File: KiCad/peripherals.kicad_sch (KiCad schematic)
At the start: 36 parts, among them IC1 MIC5350-SGYMT-TR, J1 Conn_02x06_Counter_Clockwise, J2 USB_C_Receptacle_USB2.0_14P, J3 Conn_01x07, J4 Conn_01x06, J6 Conn_02x11_Counter_Clockwise, U1 EM008LX, U2 EM008LX, U3 EM008LX, X1 2x5 0.05" SWD

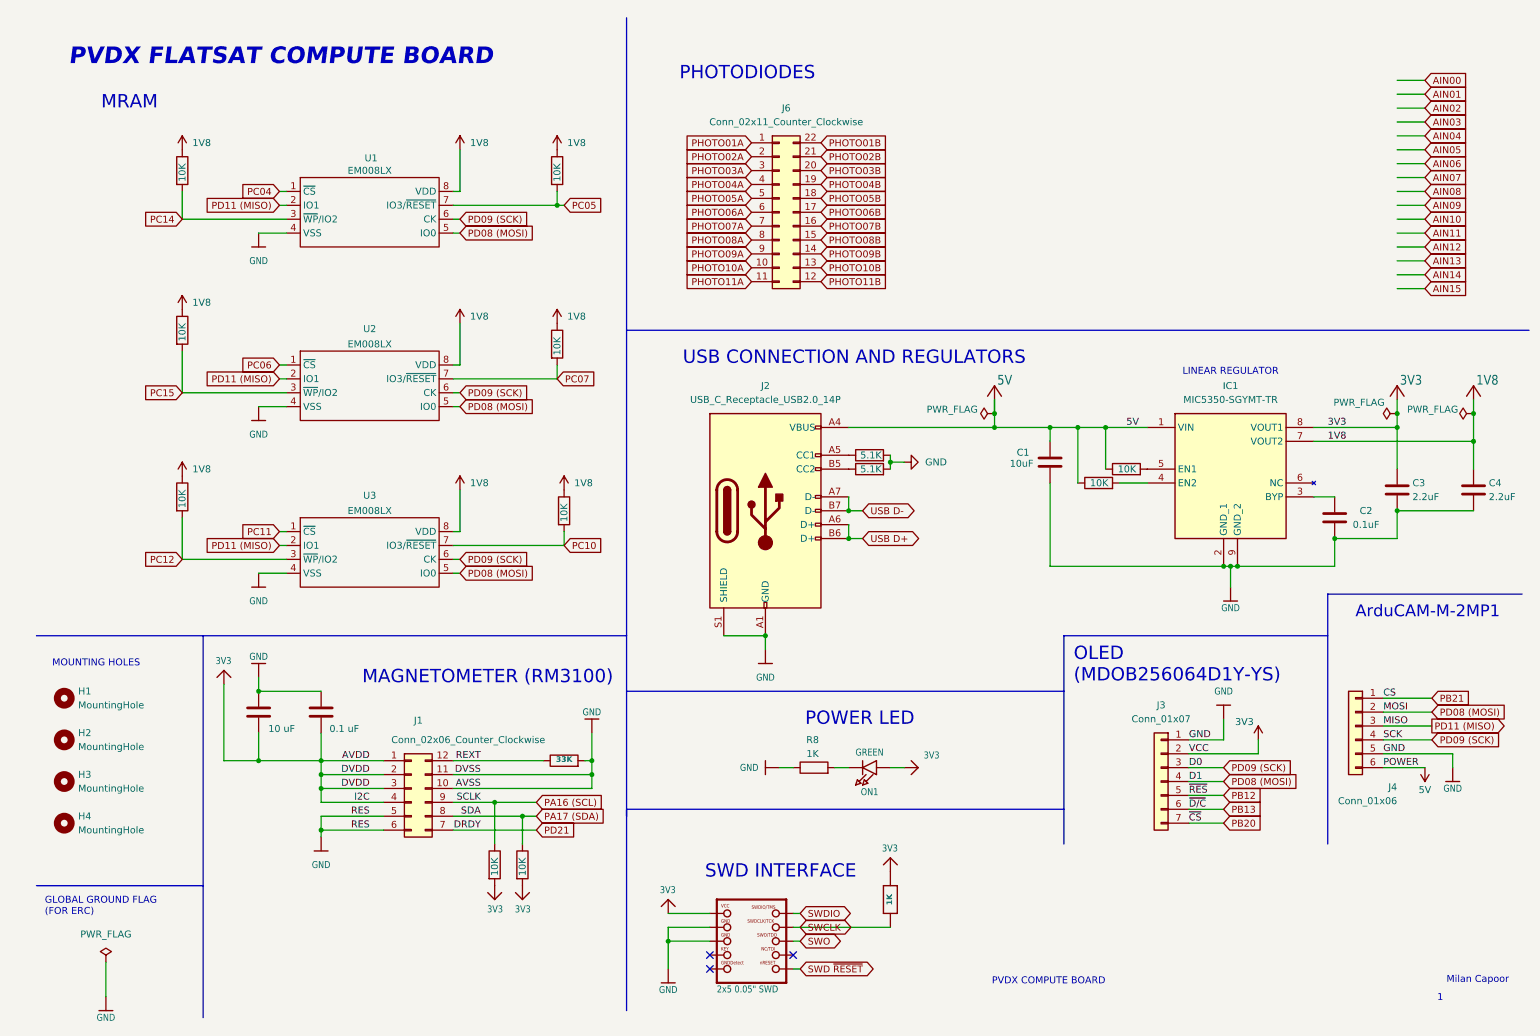
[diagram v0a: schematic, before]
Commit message: update draft to 11/13 version
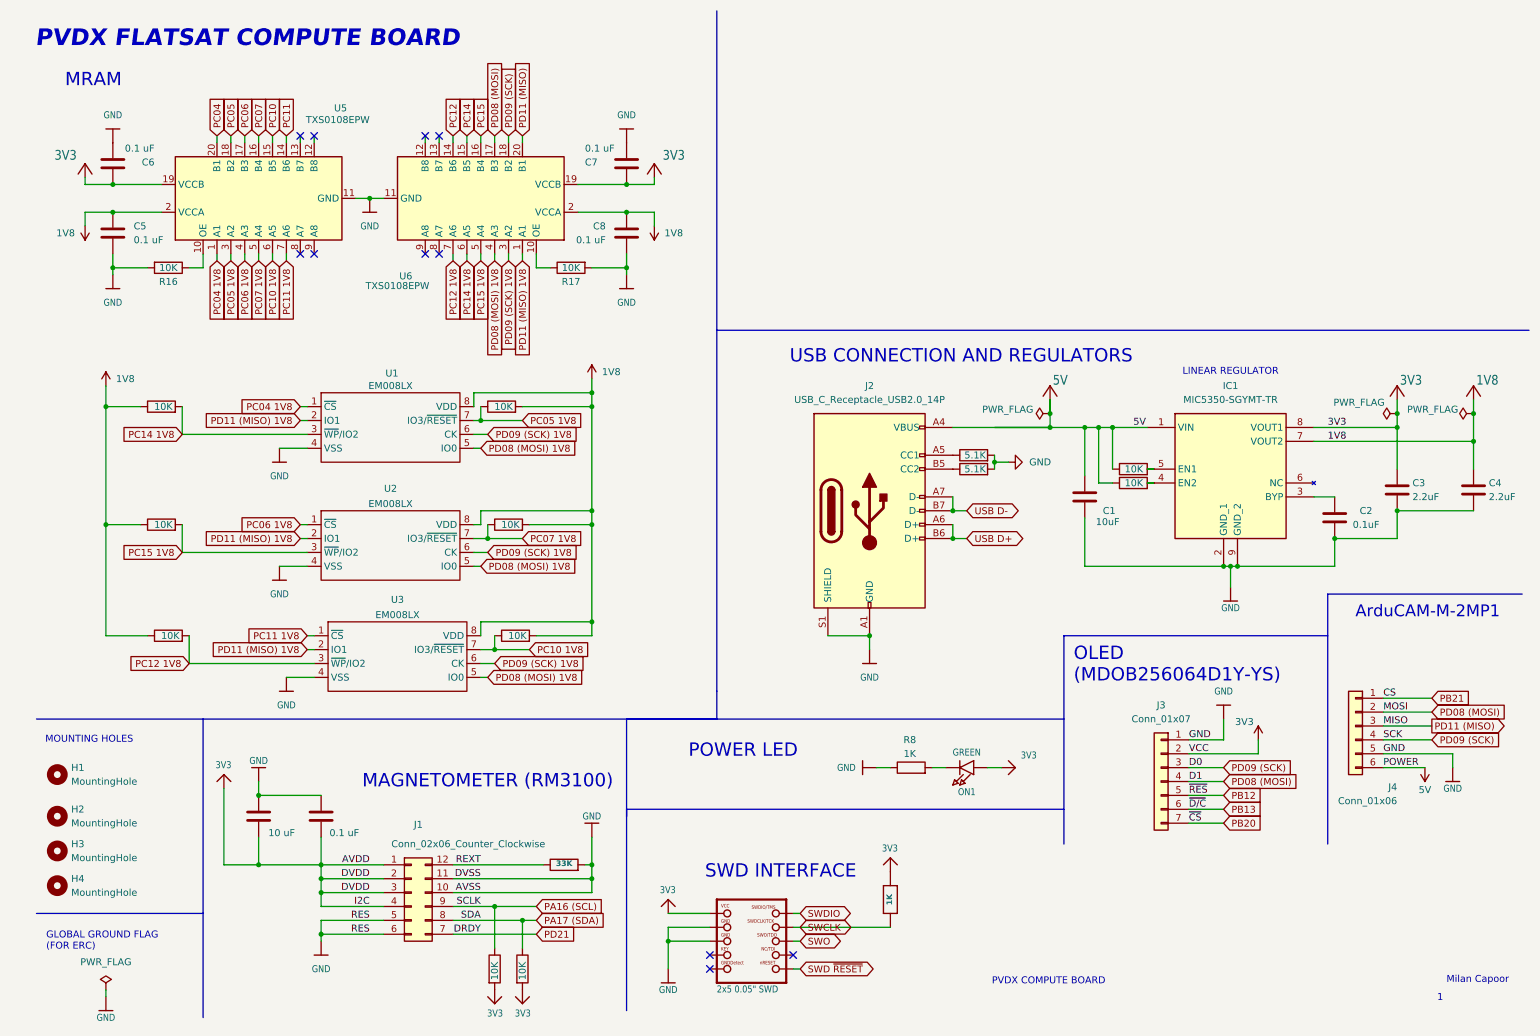
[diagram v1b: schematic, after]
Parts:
- removed J6: Conn_02x11_Counter_Clockwise, Connector_Hirose:Hirose_DF11-22DP-2DSA_2x11_P2.00mm_Vertical, symbol Connector_Generic:Conn_02x11_Counter_Clockwise
- added C5, C6, C7, C8: 0.1 uF, Capacitor_SMD:C_0201_0603Metric, symbol Device:C
- added R16, R17: 10K, Resistor_SMD:R_0603_1608Metric, symbol Device:R
- added U5, U6: TXS0108EPW, Package_SO:TSSOP-20_4.4x6.5mm_P0.65mm, symbol Logic_LevelTranslator:TXS0108EPW
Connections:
- net 1V8: now also R4.2, R5.2, R6.2, C5.1, C8.1, U5.2 (VCCA), U6.2 (VCCA); no longer R4.1, R5.1, R6.1
- net 3V3: now also C6.1, C7.1, U5.19 (VCCB), U6.19 (VCCB)
- net GND: now also C5.2, C6.2, C7.2, C8.2, R16.2, R17.2, U5.11 (GND), U6.11 (GND)
- net PC04: now also U5.20 (B1); no longer U1.1 (~{CS})
- net PC05: now also U5.18 (B2); no longer R4.2, U1.7 (IO3/~{RESET})
- net PC06: now also U5.17 (B3); no longer U2.1 (~{CS})
- net PC07: now also U5.16 (B4); no longer R5.2, U2.7 (IO3/~{RESET})
- net PC10: now also U5.15 (B5); no longer R6.2, U3.7 (IO3/~{RESET})
- net PC11: now also U5.14 (B6); no longer U3.1 (~{CS})
- net PC12: now also U6.14 (B6); no longer R3.2, U3.3 (~{WP}/IO2)
- net PC14: now also U6.15 (B5); no longer R1.2, U1.3 (~{WP}/IO2)
- net PC15: now also U6.16 (B4); no longer R2.2, U2.3 (~{WP}/IO2)
- net PD08 (MOSI): now also U6.17 (B3); no longer U1.5 (IO0), U2.5 (IO0), U3.5 (IO0)
- net PD09 (SCK): now also U6.18 (B2); no longer U1.6 (CK), U2.6 (CK), U3.6 (CK)
- net PD11 (MISO): now also U6.20 (B1); no longer U1.2 (IO1), U2.2 (IO1), U3.2 (IO1)
- new net: R16.1, U5.10 (OE)
- new net: R17.1, U6.10 (OE)
- new net PC04 1V8: U1.1 (~{CS}), U5.1 (A1)
- new net PC05 1V8: R4.1, U1.7 (IO3/~{RESET}), U5.3 (A2)
- new net PC06 1V8: U2.1 (~{CS}), U5.4 (A3)
- new net PC07 1V8: R5.1, U2.7 (IO3/~{RESET}), U5.5 (A4)
- new net PC10 1V8: R6.1, U3.7 (IO3/~{RESET}), U5.6 (A5)
- new net PC11 1V8: U3.1 (~{CS}), U5.7 (A6)
- new net PC12 1V8: R3.2, U3.3 (~{WP}/IO2), U6.7 (A6)
- new net PC14 1V8: R1.2, U1.3 (~{WP}/IO2), U6.6 (A5)
- new net PC15 1V8: R2.2, U2.3 (~{WP}/IO2), U6.5 (A4)
- new net PD08 (MOSI) 1V8: U1.5 (IO0), U2.5 (IO0), U3.5 (IO0), U6.4 (A3)
- new net PD09 (SCK) 1V8: U1.6 (CK), U2.6 (CK), U3.6 (CK), U6.3 (A2)
- new net PD11 (MISO) 1V8: U1.2 (IO1), U2.2 (IO1), U3.2 (IO1), U6.1 (A1)
- no-connect marks 3 -> 11
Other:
- note removed: "PHOTODIODES"
- moved on the sheet: C1, H1, H2, H3, H4, J1, J2, ON1, R8, U1, U2, U3
